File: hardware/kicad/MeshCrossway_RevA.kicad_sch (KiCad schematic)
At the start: 40 parts, among them J1 Waveshare ESP32-S3-Touch-LCD-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, J2 HOST DEBUG, J5 BATTERY JST-PH 2.0, U1 LOCAL 5V SOURCE — TBD, U2 XIAO + Wio-SX1262, U3 XIAO + Wio-SX1262, U4 Uputronics MAX-M10S 3V

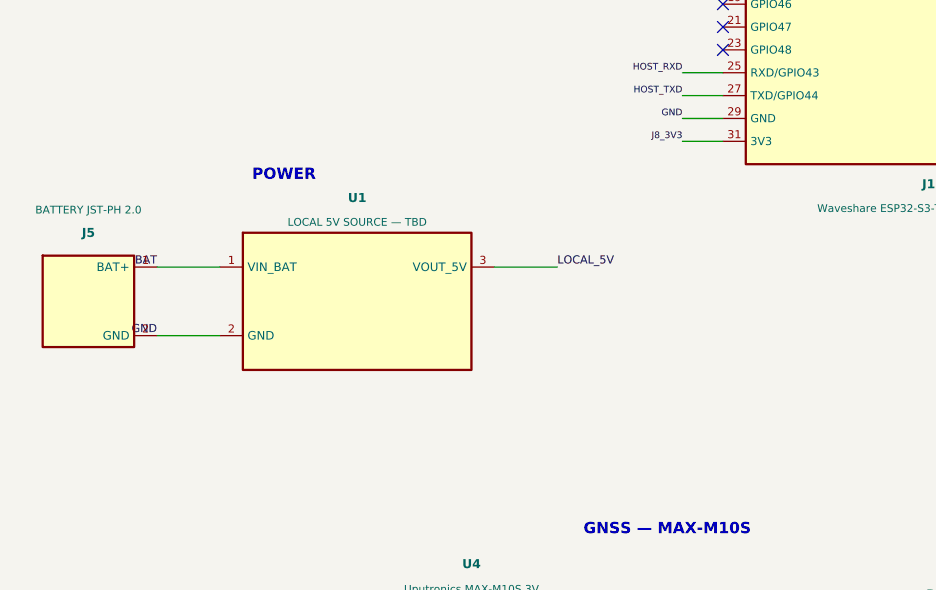
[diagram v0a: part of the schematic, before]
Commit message: Update Rev A KiCad PCB schematic and validated footprints
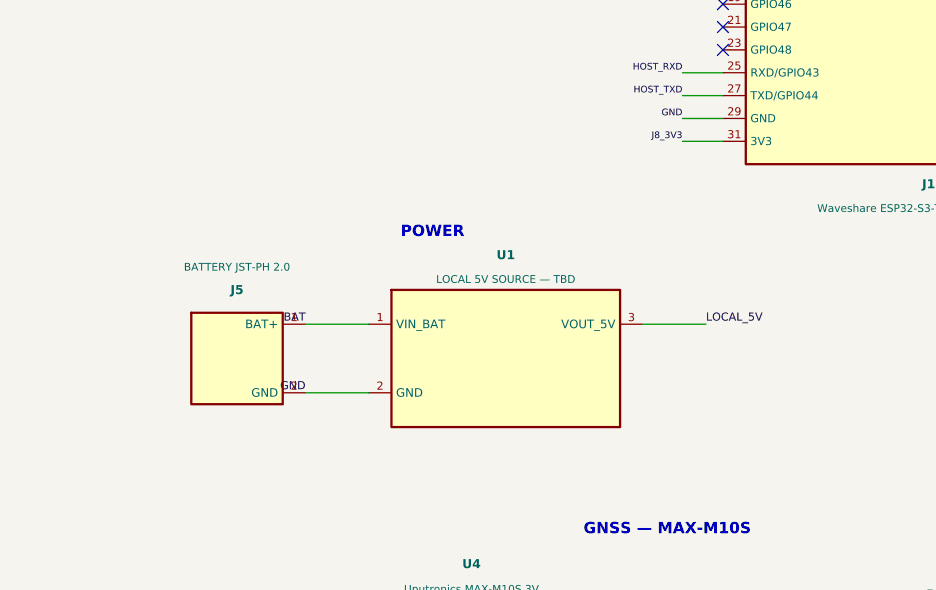
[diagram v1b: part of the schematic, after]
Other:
- moved on the sheet: J5, U1
